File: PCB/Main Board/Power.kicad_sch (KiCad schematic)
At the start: 10 parts, among them J1 Conn_01x03_Pin, U4 ${SIM.PARAMS}, U5 MIC5205-3.3YM5

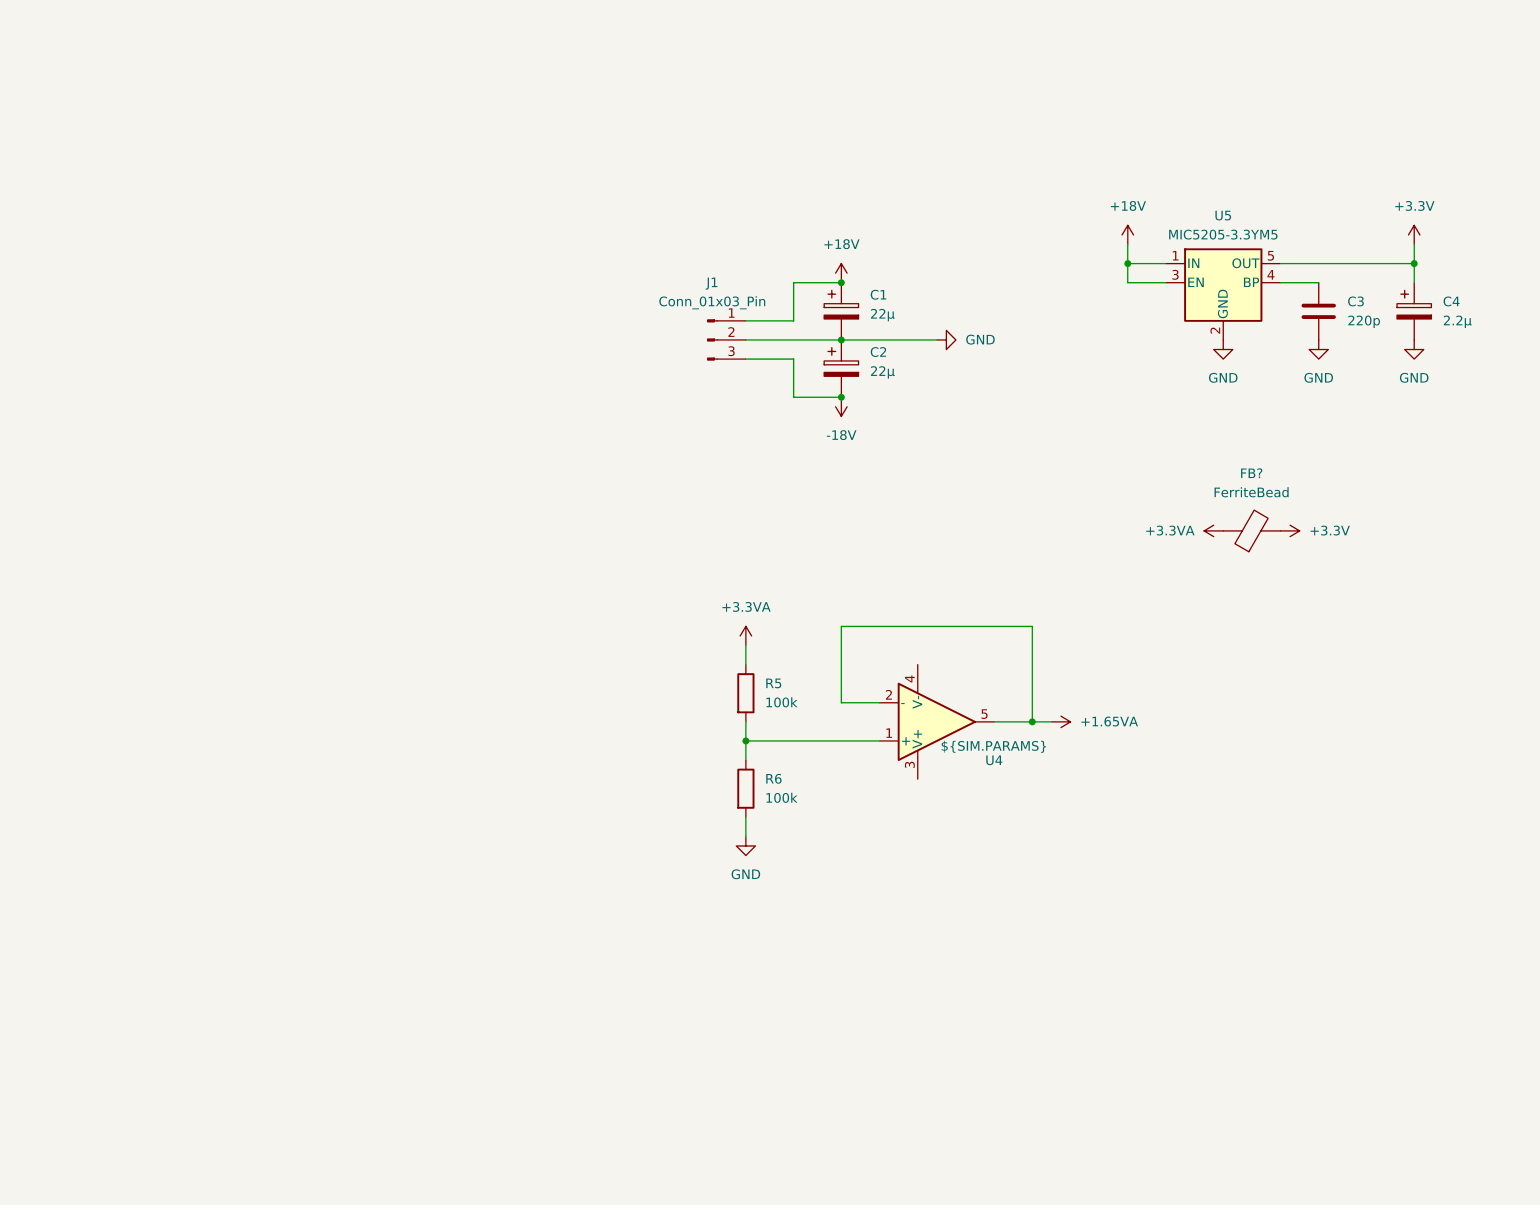
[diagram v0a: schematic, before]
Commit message: power supply
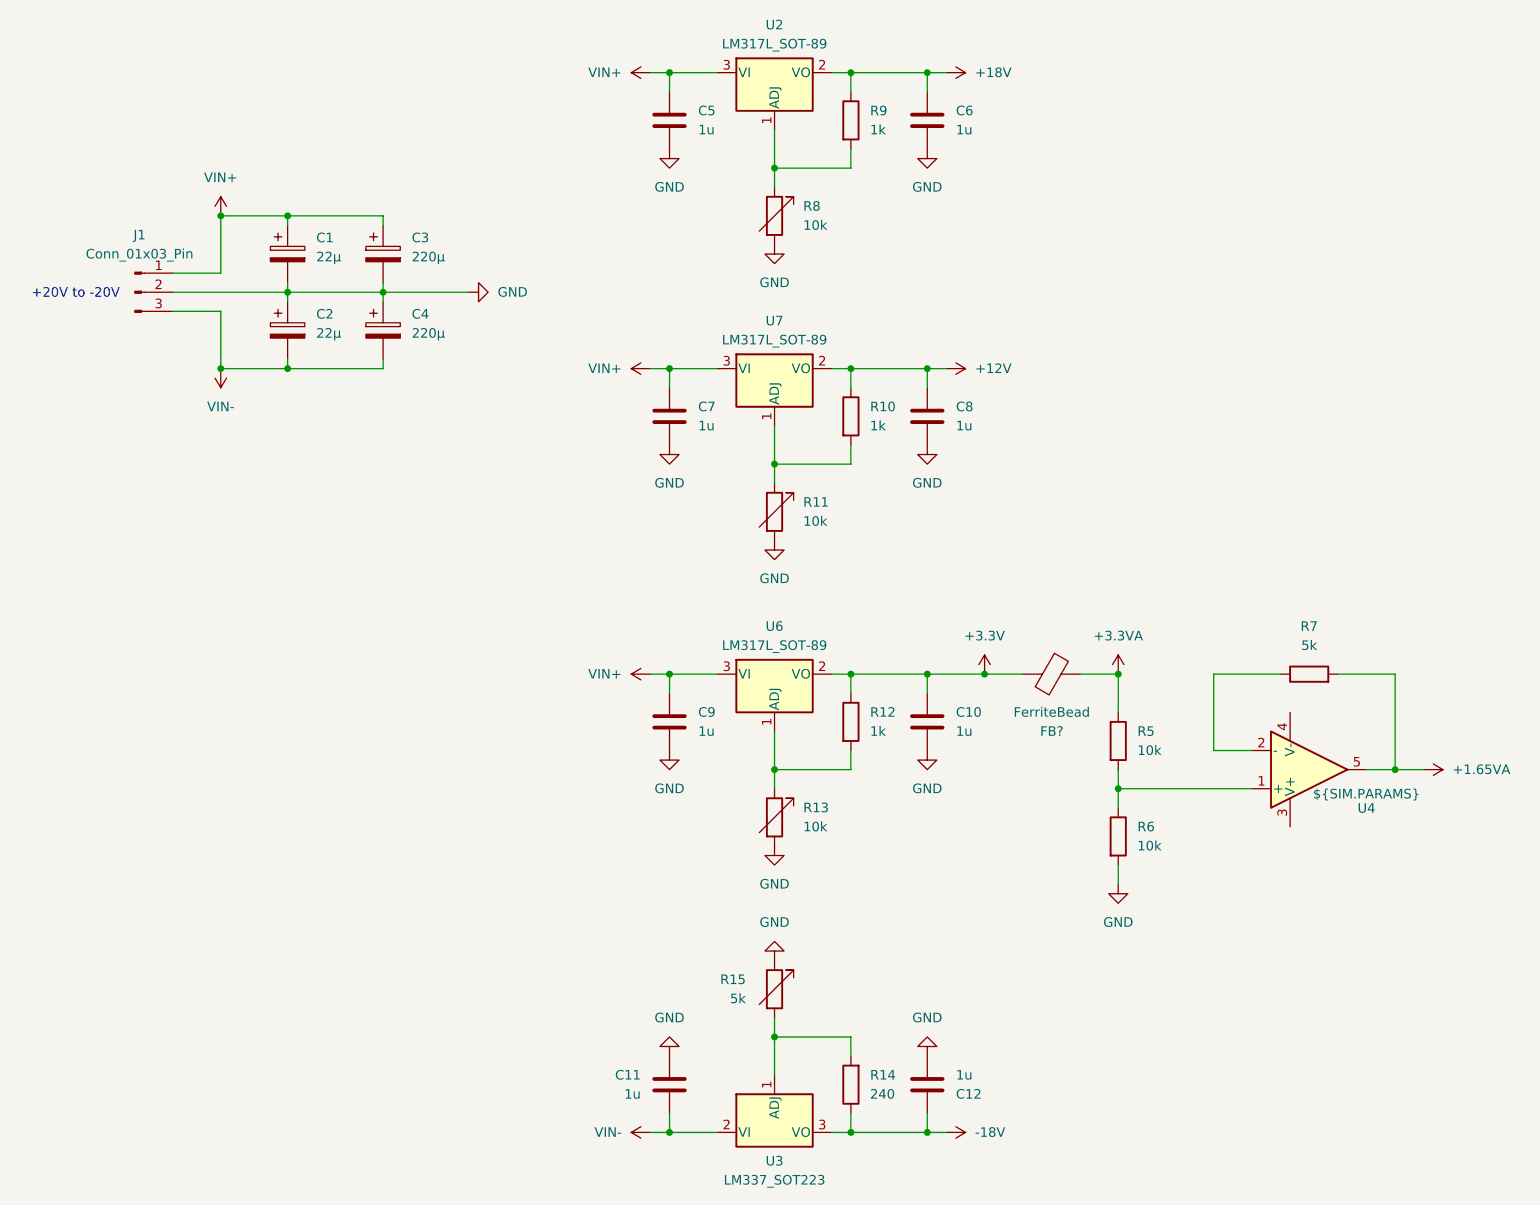
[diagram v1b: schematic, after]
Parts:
- removed C3: 220p, symbol Device:C
- removed U5: MIC5205-3.3YM5, Package_TO_SOT_SMD:SOT-23-5, symbol Regulator_Linear:MIC5205-3.6YM5
- added C10, C11, C12, C5, C6, C7, C8, C9: 1u, symbol Device:C
- added C3: 220µ, symbol Device:C_Polarized
- added R10, R12, R9: 1k, symbol Device:R
- added R11, R13, R8: 10k, symbol Device:R_Variable
- added R14: 240, symbol Device:R
- added R15: 5k, symbol Device:R_Variable
- added R7: 5k, symbol Device:R
- added U2, U6, U7: LM317L_SOT-89, Package_TO_SOT_SMD:SOT-89-3, symbol Regulator_Linear:LM317L_SOT-89
- added U3: LM337_SOT223, Package_TO_SOT_SMD:SOT-223-3_TabPin2, symbol Regulator_Linear:LM337_SOT223
- C4: value 2.2µ -> 220µ
- R5, R6: value 100k -> 10k
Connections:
- net +1.65VA: now also R7.2; no longer U4.2 (-)
- net +18V: now also C6.1, R9.1, U2.2 (VO); no longer C1.1, J1.1 (Pin_1)
- net +3.3V: now also C10.1, R12.1, U6.2 (VO); no longer C4.1
- net -18V: now also C12.1, R14.1, U3.3 (VO); no longer C2.2, J1.3 (Pin_3)
- net GND: now also C4.1, C10.2, C11.2, C12.2, C3.2, C5.2, C6.2, C7.2, C8.2, C9.2, R11.2, R13.2, R15.1, R8.2; no longer C4.2
- new net: R7.1, U4.2 (-)
- new net: R10.2, R11.1, U7.1 (ADJ)
- new net: R14.2, R15.2, U3.1 (ADJ)
- new net: R12.2, R13.1, U6.1 (ADJ)
- new net: R8.1, R9.2, U2.1 (ADJ)
- new net +12V: C8.1, R10.1, U7.2 (VO)
- new net VIN+: C1.1, C3.1, C5.1, C7.1, C9.1, J1.1 (Pin_1), U2.3 (VI), U6.3 (VI), U7.3 (VI)
- new net VIN-: C11.1, C2.2, C4.2, J1.3 (Pin_3), U3.2 (VI)
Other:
- note added: "+20V to -20V"
- moved on the sheet: C1, C2, FB?, J1, R5, R6, U4
